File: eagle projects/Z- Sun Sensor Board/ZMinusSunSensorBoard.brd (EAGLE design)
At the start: 91 x 91 mm, 194 parts, among them J2 HIROSE_FH19C-6S-0.5SH(10), J3 HIROSE_FH19C-6S-0.5SH(10), J4 HIROSE_FH19C-6S-0.5SH(10), J5 HIROSE_FH19C-6S-0.5SH(10), U1 ADS7841E_2K5, U13 ADS7841E_2K5, U15 TLV9051IDCKR, U19 TLV9051IDCKR, U2 ADS7841E_2K5, U21 TLV9051IDCKR, U23 TLV9051IDCKR, U24 TLV9051IDCKR, U25 ADS7841E_2K5, U26 TLV9051IDCKR, U27 ADS7841E_2K5, U28 TLV9051IDCKR, U29 TLV9051IDCKR, U3 TLV9051IDCKR, U30 TLV9051IDCKR, U31 TLV9051IDCKR, U32 TLV9051IDCKR, U4 LM20BIM7X_NOPB, U6 TLV9051IDCKR, U8 TLV9051IDCKR, U9 TLV9051IDCKR

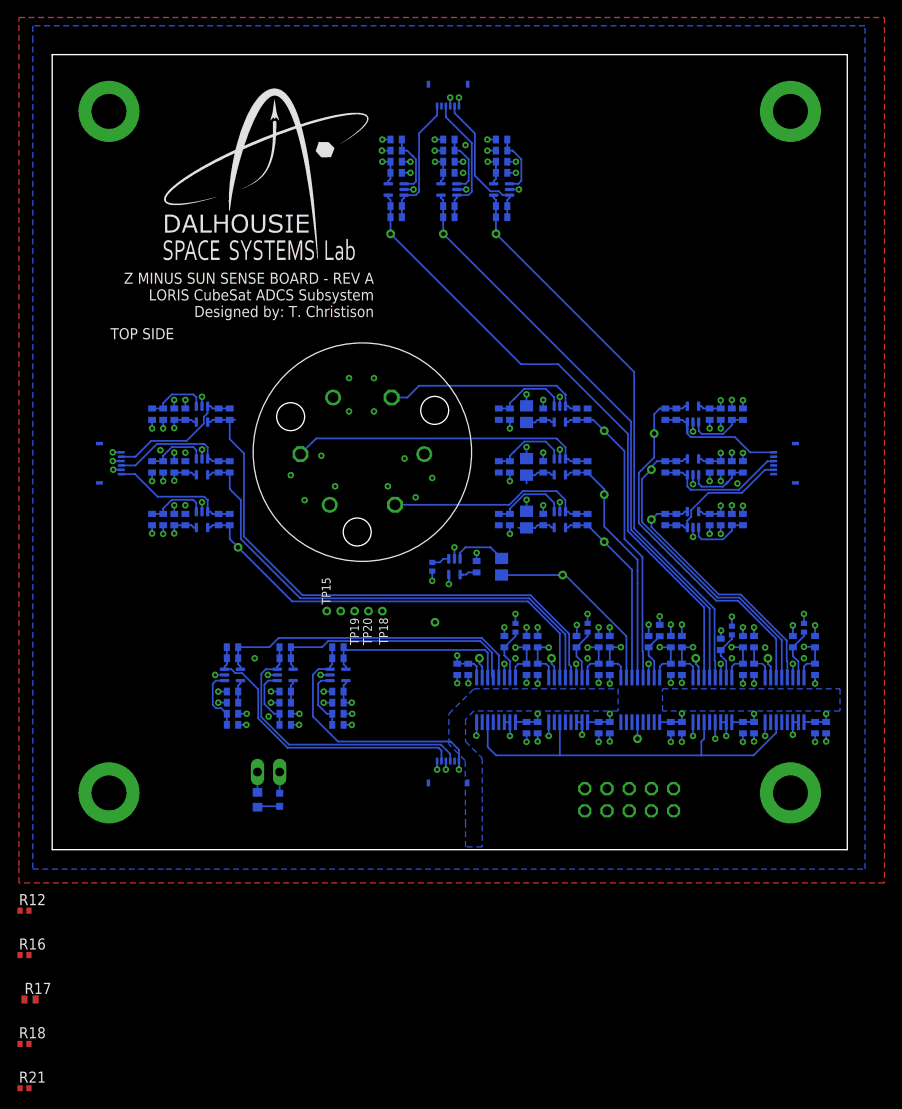
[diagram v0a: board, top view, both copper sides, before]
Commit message: Rev B almost ready
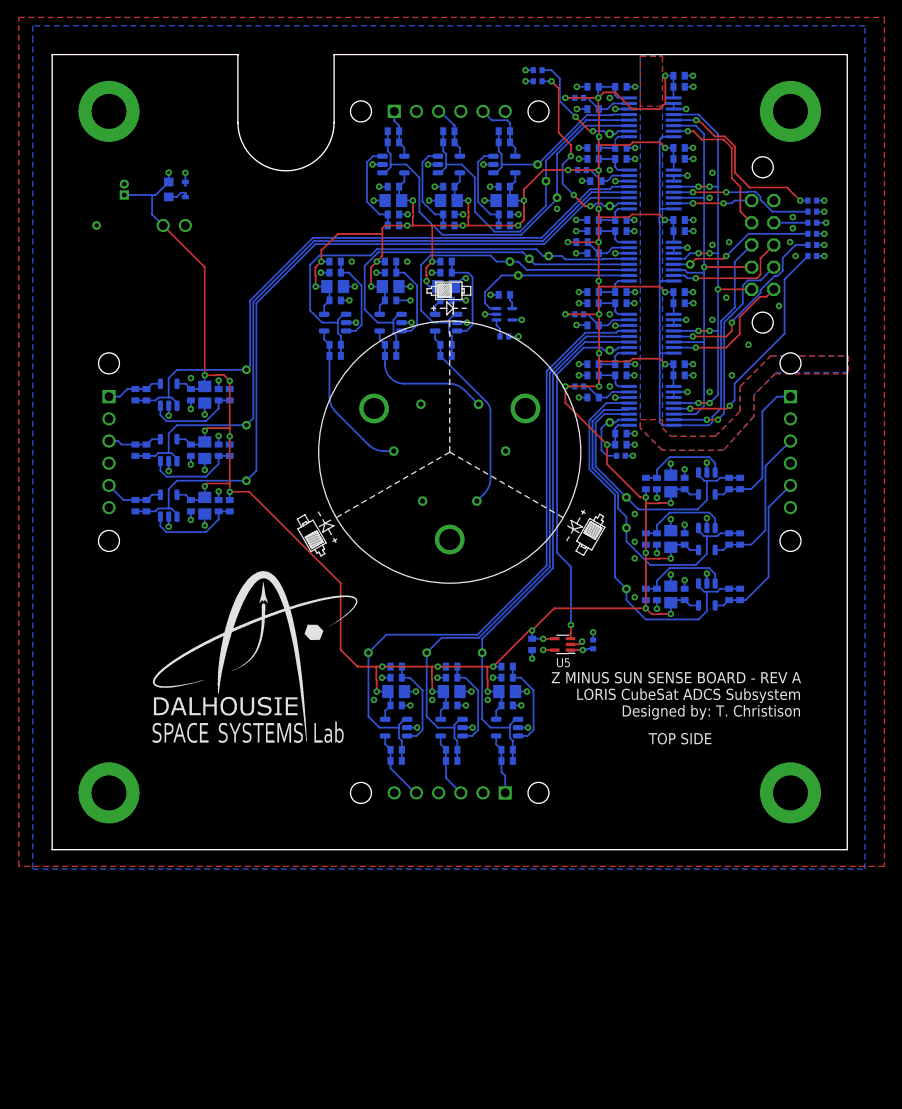
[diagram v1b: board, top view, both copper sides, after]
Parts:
- removed A1: XY_SUN_SENSOR, my_library:XY_SUN_SENOR_MASK
- removed C104, C107, C109, C112, C114, C31, C69, C86, C97: 0.1u, resistor:C0402
- removed C105, C110, C111, C115, C116, C33, C54, C70, C84, C98: 0.022u, resistor:C0402
- removed C106, C108, C113, C55, C68, C85, C99: 4.7u, resistor:C0402
- removed C30: 4.7u, rcl:C0805
- removed J4, J5: HIROSE_FH19C-6S-0.5SH(10), my_library:HIROSE_FH19C-6S-0.5SH(10)
- removed JP1: (no value), pinhead:1X02
- removed JP3: (no value), pinhead:2X05
- removed R2: 0R, rcl:R0805
- removed R28, R57, R63, R69: 13.7k, resistor:R0402
- removed R31, R46, R55, R61, R67: 3.74k, resistor:R0402
- removed R56, R62, R68: 280R, resistor:R0402
- removed TP12, TP18, TP20, TP7, TP8: TESTPOINT, my_library:TP_P76H50
- removed U15, U24, U28, U30, U31, U32: TLV9051IDCKR, my_library:SC70-5P65_210X110L36X22N_TLV9051
- added C10, C17, C24, C36, C39, C4, C58, C64, C7: 0.1u, resistor:C0402
- added C11, C18, C34, C37, C40, C5, C59, C8: 0.022u, resistor:C0402
- added C13, C23, C3, C35, C38, C44, C57, C6, C63, C9: 4.7u, rcl:C0805
- added C2: 0.1u, rcl:C0402
- added J1: TE-1734829-2, my_library:TE-1734829-2
- added JP2, JP4, JP5, JP6: (no value), my_library:1X06_MTG_HOLES
- added R27: 5.1M, rcl:R0402
- added R30, R37, R43, R49, R71, R79: 280R, resistor:R0402
- added R35, R41, R72, R74, R80: 13.7k, resistor:R0402
- added R36, R42, R73, R75, R81: 3.74k, resistor:R0402
- added TP23, TP24, TP25, TP27, TP29: TESTPOINT, my_library:TP_P76H50
- added U$1: SSR_MOUNT_03, my_library:SSR_MOUNT_03
- added U$3, U$4, U$5: (no value), my_library:PHOTODIODE_SILK
- added U10, U11, U12, U14, U16, U17: TSV991AILT, my_library:SOT95P280X145-5N
- added U5: LM20BIM7X_NOPB, my_library:SOT23-5P65_210X110L40X22N_LM20
- C100, C71: value 0.022u -> 4.7u; device resistor:C0402 -> rcl:C0805
- C101, C27, C32: value 0.022u -> 0.1u
- C103, C96: value 4.7u -> 0.022u
- C25, C28: value 4.7u -> 0.022u; device rcl:C0805 -> resistor:C0402
- C26, C29: value 0.1u -> 4.7u; device resistor:C0402 -> rcl:C0805
- C52, C82: value 4.7u -> 0.1u
- C53, C67, C83: value 0.1u -> 0.022u
- C87: device resistor:C0402 -> rcl:C0805
- J2: value HIROSE_FH19C-6S-0.5SH(10) -> (none); device my_library:HIROSE_FH19C-6S-0.5SH(10) -> my_library:2X05
- J3: value HIROSE_FH19C-6S-0.5SH(10) -> (none); device my_library:HIROSE_FH19C-6S-0.5SH(10) -> my_library:1X02
- LED1: device led:CHIP-LED0603 -> led:CHIPLED-0603-TTW
- R14, R25: value 280R -> 5.1M; device resistor:R0402 -> rcl:R0402
- R15: value 13.7k -> 5.1M; device resistor:R0402 -> rcl:R0402
- R17: device resistor:R0402 -> rcl:R0402
- R19: value 3.74k -> 5.1M; device resistor:R0402 -> rcl:R0402
- R44, R53, R59, R65: value 280R -> 13.7k
- R45, R54, R60, R66: value 13.7k -> 3.74k
- R58, R64, R70: value 3.74k -> 280R
- U19, U21, U23, U26, U29, U3, U6, U8, U9: value TLV9051IDCKR -> TSV991AILT; device my_library:SC70-5P65_210X110L36X22N_TLV9051 -> my_library:SOT95P280X145-5N
- moved R21 134.9 mm to (87.0, 73.0), flipped to the bottom
- moved R18 127.5 mm to (87.0, 67.9), flipped to the bottom
- moved R17 125.3 mm to (87.0, 70.5), flipped to the bottom
- moved R12 121.4 mm to (87.0, 74.3), flipped to the bottom
- moved R16 121.4 mm to (87.0, 69.2), flipped to the bottom
- moved J2 78.7 mm to (81.3, 69.2)
- moved C50 76.5 mm to (71.8, 88.6), turned to 180 degrees
- moved C49 75.0 mm to (71.8, 87.3), turned to 180 degrees
- moved J3 75.0 mm to (14.0, 71.4), turned to 180 degrees
- moved LED1 70.7 mm to (15.2, 75.6)
- moved R11 70.6 mm to (13.3, 75.6)
- moved C46 70.3 mm to (65.1, 87.3), turned to 180 degrees
- moved R60 69.2 mm to (77.5, 29.2), turned to 90 degrees
- moved U13 68.4 mm to (68.6, 83.8), turned to 180 degrees
- moved C45 68.4 mm to (61.9, 87.3), turned to 0 degrees
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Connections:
- removed net !CS!_SUN_Z+: U2.15
- removed net N$1: R2.1, U4.3
- removed net N$13: R14.2, R15.1, U9.1
- removed net N$3: A1.C1, C27.1, R7.1, U6.3
- removed net N$31: R22.2, R23.1, U3.1
- removed net N$34: R25.2, R28.1, U23.1
- removed net N$36: R32.2, R33.1, U24.1
- removed net N$45: R44.2, R45.1, U19.1
- removed net N$47: R50.2, R51.1, U21.1
- removed net N$48: LED1.A, R11.1
- removed net N$5: TP17.1, U25.2
- removed net N$56: R56.2, R57.1, U28.1
- removed net N$58: R59.2, R60.1, U29.1
- removed net N$64: R65.2, R66.1, U31.1
- removed net N$66: R68.2, R69.1, U32.1
- removed net N$68: JP3.10
- removed net N$9: R8.2, R9.1, U8.1
- removed net TEMP: R2.2, TP1.1, U2.2
- new net N$20: R27.1, U5.1
- new net N$21: LED1.A@1, R11.1
- new net N$27: C8.1, R13.1, U$1.C2, U8.4
- new net N$28: R8.2, R9.1, U8.3
- new net N$30: R43.2, R44.1, U12.3
- new net N$32: R22.2, R23.1, U3.3
- new net N$40: R30.2, R35.1, U9.3
- new net N$42: C18.1, R42.1, U$1.C1, U11.4
- new net N$43: R37.2, R41.1, U11.3
- new net N$60: R49.2, R53.1, U14.3
- new net N$69: R64.2, R65.1, U23.3
- new net N$71: R71.2, R72.1, U17.3
- new net N$74: R70.2, R74.1, U26.3
- new net N$78: R79.2, R80.1, U29.3
- new net TEMP_EXT: TP17.1, U25.2, U5.3
- new net TEMP_INT: TP1.1, U2.2, U4.3
- net !CS!_SUN_X+: now also J2.2; no longer JP3.2
- net !CS!_SUN_X-: now also J2.7; no longer JP3.7
- net !CS!_SUN_Y+: now also J2.4; no longer JP3.4
- net !CS!_SUN_Y-: now also J2.9; no longer JP3.9
- net !CS!_SUN_Z-: now also J2.6, U2.15; no longer JP3.6
- net +3V3: now also C10.1, C100.1, C101.1, C13.1, C17.1, C2.1, C23.1, C24.1, C27.1, C3.1, C32.1, C35.1, C36.1, C38.1, C39.1, C4.1, C44.1, C57.1, C58.1, C6.1, C63.1, C64.1, C7.1, C71.1, C9.1, J1.1, J2.10, J3.1, R35.2, R41.2, R44.2, R53.2, R59.2, R65.2, R72.2, R74.2, R80.2, U10.5, U11.5, U12.5, U14.5, U16.5, U17.5, U5.4; no longer C103.1, C104.1, C106.1, C107.1, C108.1, C109.1, C112.1, C113.1, C114.1, C25.1, C28.1, C30.1, C31.1, C53.1, C55.1, C67.1, C68.1, C69.1, C83.1, C85.1, C86.1, C96.1, C97.1, C99.1, JP1.1, R15.2, R28.2, R45.2, R54.2, R57.2, R60.2, R63.2, R66.2, R69.2, U15.5, U24.5, U28.5, U30.5, U31.5, U32.5
- net 0_DEGREES: now also C18.2, R42.2, TP24.1, U11.1; no longer C27.2, R7.2, TP3.1, U6.4
- net 120_DEGREES: now also C8.2, U8.1; no longer C32.2, U8.4
- net 240_DEGREES: now also C5.2, R7.2, TP3.1, U6.1; no longer C33.2, R19.2, TP8.1, U9.4
- net GND: now also C10.2, C100.2, C101.2, C13.2, C17.2, C2.2, C23.2, C24.2, C27.2, C3.2, C32.2, C35.2, C36.2, C38.2, C39.2, C4.2, C44.2, C57.2, C58.2, C6.2, C63.2, C64.2, C7.2, C71.2, C9.2, J1.2, JP2.2, JP2.4, JP2.6, JP4.2, JP4.4, JP4.6, JP5.2, JP5.4, JP5.6, JP6.2, JP6.4, JP6.6, LED1.C@1, R15.1, R19.1, R25.2, R27.2, R30.1, R37.1, R43.1, R49.1, R58.1, R64.1, R70.1, R71.1, R79.1, U$1.A1, U$1.A2, U$1.A3, U10.2, U11.2, U12.2, U14.2, U16.2, U17.2, U5.2, U5.5; no longer A1.A1, A1.A2, A1.A3, C103.2, C104.2, C106.2, C107.2, C108.2, C109.2, C112.2, C113.2, C114.2, C25.2, C28.2, C30.2, C31.2, C53.2, C55.2, C67.2, C68.2, C69.2, C83.2, C85.2, C86.2, C96.2, C97.2, C99.2, J2.2, J2.4, J2.6, J2.7, J2.8, J3.4, J3.6, J3.7, J3.8, J4.2, J4.4, J4.6, J4.7, J4.8, J5.2, J5.4, J5.6, J5.7, J5.8, JP1.2, LED1.C, R25.1, R44.1, R53.1, R56.1, R59.1, R62.1, R65.1, R68.1, U15.2, U24.2, U28.2, U30.2, U31.2, U32.2
- net N$10: now also R15.2
- net N$11: now also R14.2
- net N$12: now also C5.1, R7.1, U$1.C3, U6.4; no longer A1.C3, C33.1, R19.1, U9.3
- net N$14: now also R19.2
- net N$23: now also C96.1, JP6.3, R75.1, U26.4; no longer C100.1, J5.3, R31.1, U23.3
- net N$29: now also C83.1, JP6.1, R66.1, U23.4; no longer C84.1, J5.1, R24.1, U3.3
- net N$35: now also C103.1, JP6.5, R81.1, U29.4; no longer C101.1, J5.5, R34.1, U24.3
- net N$37: now also C34.1, JP5.1, R45.1, U12.4; no longer C98.1, J4.1, R64.1, U30.3
- net N$38: now also C25.1, JP4.1, U10.4; no longer C54.1, J3.1, U15.3
- net N$41: now also R32.2, R33.1, U16.3; no longer R38.2, R39.1, U15.1
- net N$44: now also C40.1, JP4.3, R24.1, U3.4; no longer C70.1, J3.3, R46.1, U19.3
- net N$46: now also C53.1, JP4.5, R34.1, U16.4; no longer C71.1, J3.5, R52.1, U21.3
- net N$49: now also C11.1, JP2.1, R36.1, U9.4; no longer C105.1, J2.1, R55.1, U26.3
- net N$54: now also R50.2, R51.1, U19.3; no longer R53.2, R54.1, U26.1
- net N$55: now also C28.1, JP2.3, R54.1, U14.4; no longer C110.1, J2.3, R58.1, U28.3
- net N$57: now also C37.1, JP2.5, R73.1, U17.4; no longer C111.1, J2.5, R61.1, U29.3
- net N$6: now also R38.2, R39.1, U10.3; no longer R1.2, R3.1, U6.1
- net N$61: now also R58.2, R59.1, U21.3; no longer R62.2, R63.1, U30.1
- net N$63: now also C59.1, JP5.3, R52.1, U19.4; no longer C115.1, J4.3, R67.1, U31.3
- net N$65: now also C67.1, JP5.5, R60.1, U21.4; no longer C116.1, J4.5, R70.1, U32.3
- net N$67: now also J2.8, R25.1; no longer JP3.8
- net N$8: now also R1.2, R3.1, U6.3; no longer A1.C2, C32.1, R13.1, U8.3
- net UCB0_SPI_CLK: now also J2.5; no longer JP3.5
- net UCB0_SPI_MISO: now also J2.1; no longer JP3.1
- net UCB0_SPI_MOSI: now also J2.3; no longer JP3.3
- net X+_0_DEGREES: now also C11.2, R36.2, U9.1; no longer C105.2, R55.2, U26.4
- net X+_120_DEGREES: now also C28.2, R54.2, TP16.1, U14.1; no longer C110.2, R58.2, TP15.1, U28.4
- net X+_240_DEGREES: now also C37.2, R73.2, TP25.1, U17.1; no longer C111.2, R61.2, TP16.1, U29.4
- net X-_0_DEGREES: now also C25.2, U10.1; no longer C54.2, U15.4
- net X-_120_DEGREES: now also C40.2, R24.2, TP5.1, U3.1; no longer C70.2, R46.2, TP11.1, U19.4
- net X-_240_DEGREES: now also C53.2, R34.2, TP9.1, U16.1; no longer C71.2, R52.2, TP12.1, U21.4
- net Y+_0_DEGREES: now also C34.2, R45.2, TP11.1, U12.1; no longer C98.2, R64.2, TP18.1, U30.4
- net Y+_120_DEGREES: now also C59.2, R52.2, TP15.1, U19.1; no longer C115.2, R67.2, TP19.1, U31.4
- net Y+_240_DEGREES: now also C67.2, R60.2, TP19.1, U21.1; no longer C116.2, R70.2, TP20.1, U32.4
- net Y-_0_DEGREES: now also C103.2, R81.2, TP29.1, U29.1; no longer C84.2, R24.2, TP5.1, U3.4
- net Y-_120_DEGREES: now also C96.2, R75.2, TP27.1, U26.1; no longer C100.2, R31.2, TP7.1, U23.4
- net Y-_240_DEGREES: now also C83.2, R66.2, TP23.1, U23.1; no longer C101.2, R34.2, TP9.1, U24.4
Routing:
- net +3V3: track 149.7 -> 488.3 mm, vias 42 -> 53
- net UCB0_SPI_CLK: track 6.65 -> 67.4 mm, vias 4 -> 0
- net UCB0_SPI_MISO: track 1.89 -> 60.6 mm, vias 1 -> 9
- net TEMP_EXT: track 0.00 -> 40.7 mm, vias 0 -> 1
- net N$3: track 35.5 -> 0.00 mm
- net N$52: track 0.00 -> 27.5 mm, vias 0 -> 2
- net !CS!_SUN_Y+: track 0.00 -> 26.0 mm, vias 0 -> 2
- net TEMP: track 21.9 -> 0.00 mm
- net N$50: track 0.00 -> 21.4 mm, vias 0 -> 2
- net N$51: track 0.00 -> 21.4 mm, vias 0 -> 2
- net N$14: track 2.34 -> 23.2 mm, vias 0 -> 4
- net TEMP_INT: track 0.00 -> 20.1 mm
- net N$27: track 0.00 -> 18.0 mm, vias 1 -> 0
- net 0_DEGREES: track 28.5 -> 45.9 mm
- net 240_DEGREES: track 22.2 -> 39.4 mm
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- added copper zone on layer 15, net +3V10
- added copper zone on layer 15, net +3V11
- added copper zone on layer 15, net +3V12
- added copper zone on layer 15, net +3V14
- added copper zone on layer 15, net +3V16
- added copper zone on layer 15, net +3V18
- added copper zone on layer 15, net +3V20
- added copper zone on layer 15, net +3V22
- added copper zone on layer 15, net +3V24
- added copper zone on layer 15, net +3V4
- added copper zone on layer 15, net +3V5
- added copper zone on layer 15, net +3V6
- added copper zone on layer 15, net +3V7
- added copper zone on layer 15, net +3V8
- added copper zone on layer 15, net +3V9
- added copper zone on layer 2, net GND10
- added copper zone on layer 2, net GND11
- added copper zone on layer 2, net GND13
- added copper zone on layer 2, net GND15
- added copper zone on layer 2, net GND17
- added copper zone on layer 2, net GND19
- added copper zone on layer 2, net GND21
- added copper zone on layer 2, net GND23
- added copper zone on layer 2, net GND3
- added copper zone on layer 2, net GND4
- added copper zone on layer 2, net GND5
- added copper zone on layer 2, net GND6
- added copper zone on layer 2, net GND7
- added copper zone on layer 2, net GND8
- added copper zone on layer 2, net GND9
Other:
- outline, holes or cut-outs redrawn
- board text removed: "U15"
- board text removed: "U19"
- board text removed: "U21"
- board text removed: "U23"
- board text removed: "U24"
- board text removed: "U26"
- board text removed: "U28"
- board text removed: "U29"
- board text removed: "U30"
- board text removed: "U31"
- board text removed: "U32"
- board text removed: "U6"
- board text removed: "U8"
- board text removed: "U9"
